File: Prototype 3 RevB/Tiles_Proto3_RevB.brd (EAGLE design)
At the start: 62 parts, among them Q1 DMG3415U-7, U2 MF-DSC-SOT233-MMBT3904, X1 32.768

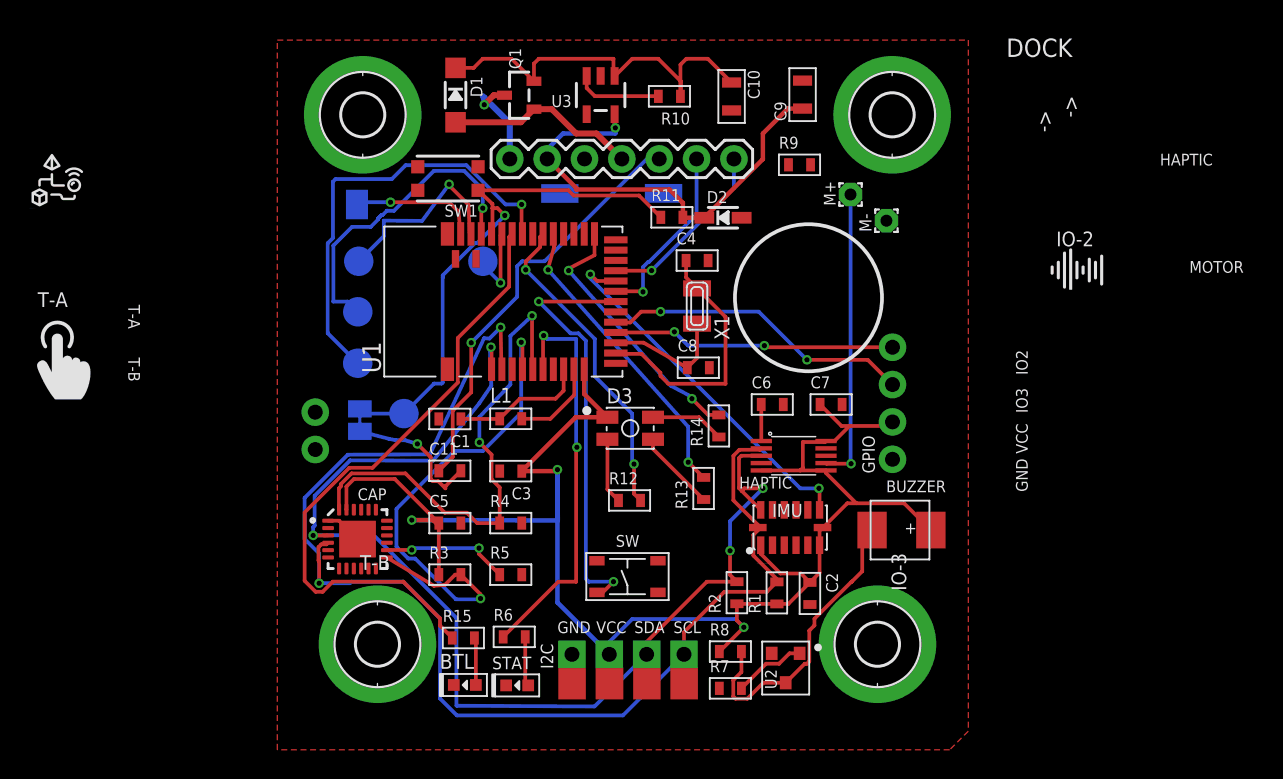
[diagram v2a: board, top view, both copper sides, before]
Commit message: ready for prod
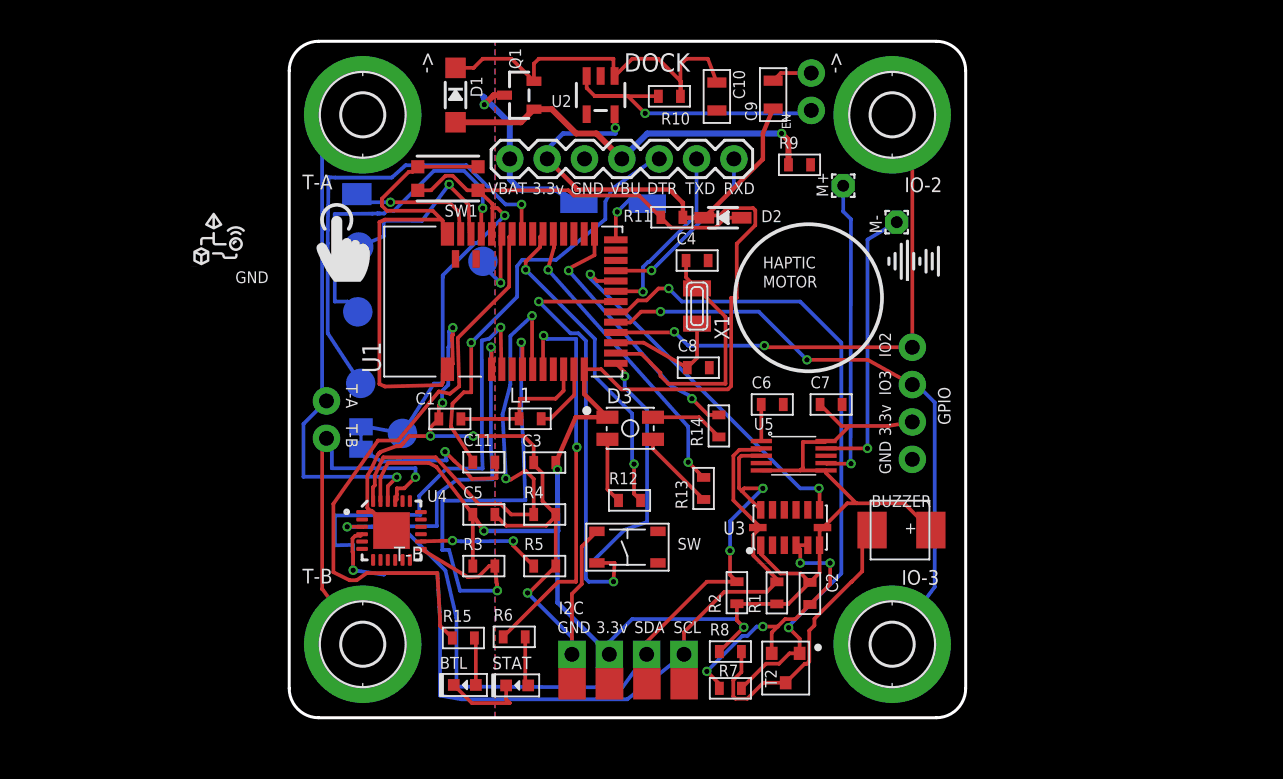
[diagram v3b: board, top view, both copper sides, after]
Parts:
- removed CAP: (no value), cap1188-microbuilder:QFN24_4MM_SMSC
- removed IMU: ADXL345BCCZ-RL, Seeed-OPL-sensor:LGA14-0.8-5.0X3.0MM
- added EN: (no value), SparkFun-Connectors:1X02_NO_SILK
- added T2: MF-DSC-SOT233-MMBT3904, MF_Discrete_Semiconductor:SOT-23-3
- added U4: CAP1188, cap1188-microbuilder:QFN24_4MM_SMSC
- U1: value (none) -> MDBT42Q
- U2: value MF-DSC-SOT233-MMBT3904 -> AP2112; device MF_Discrete_Semiconductor:SOT-23-3 -> microbuilder2:SOT23-5
- U3: value (none) -> ADXL345; device microbuilder2:SOT23-5 -> Seeed-OPL-sensor:LGA14-0.8-5.0X3.0MM
- moved U2 40.9 mm to (18.2, 1.34), turned to 180 degrees
- moved U3 32.1 mm to (31.1, -28.1), turned to 90 degrees
- moved C11 2.38 mm to (10.2, -23.6)
- moved C3 2.38 mm to (14.4, -23.6)
- moved C5 2.38 mm to (10.2, -27.2)
- moved R3 2.38 mm to (10.2, -30.7)
- moved R4 2.38 mm to (14.4, -27.2)
- moved R5 2.38 mm to (14.4, -30.7)
- moved C9 2.00 mm to (29.9, 1.37)
- moved SW 2.00 mm to (20.0, -29.4)
- moved B+ 1.47 mm to (16.7, -6.04)
- moved SWO 1.39 mm to (1.86, -18.3)
- moved RST 1.35 mm to (4.70, -21.7)
- moved GPIO 1.35 mm to (39.4, -15.8)
- moved L1 1.32 mm to (13.4, -20.7)
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- renumbered HAPTIC to U5
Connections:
- removed net N$10: R10.P$2, U3.3
- new net EN: EN.1, R10.P$2, U2.3
- net 3.3V: now also U2.5, U3.1, U3.6, U3.7, U4.23; no longer CAP.23, IMU.1, IMU.6, IMU.7, U3.5
- net BUZZER: now also T2.P$1; no longer U2.P$1
- net CAP-A: now also U4.22; no longer CAP.22
- net CAP-B: now also U4.21; no longer CAP.21
- net CAP-INT: now also U4.13; no longer CAP.13
- net CAP-RES: now also U4.24; no longer CAP.24
- net GND: now also EN.2, T2.P$2, U2.2, U3.4, U3.5, U4.1, U4.THERM; no longer CAP.1, CAP.THERM, IMU.2, IMU.4, IMU.5, U2.P$2
- net IMU-INT: now also U3.8; no longer IMU.8
- net N$13: now also U2.1; no longer U3.1
- net N$3: now also U4.14; no longer CAP.14
- net N$4: now also T2.P$3; no longer U2.P$3
- net SCL: now also U3.14, U4.4; no longer CAP.4, IMU.14
- net SDA: now also U3.13, U4.3; no longer CAP.3, IMU.13
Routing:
- net GND: track 2.52 -> 145.2 mm, vias 0 -> 11
- net BUZZER: track 4.95 -> 45.4 mm, vias 0 -> 2
- net CAP-A: track 0.00 -> 34.8 mm, vias 0 -> 1
- net CAP-B: track 0.00 -> 26.2 mm, vias 0 -> 1
- net EN: track 0.00 -> 21.2 mm, vias 0 -> 1
- net IO-3: track 21.2 -> 41.7 mm
- net N$7: track 0.00 -> 19.3 mm, vias 0 -> 1
- net 3.3V: track 143.8 -> 163.0 mm
- net IO-2: track 19.3 -> 37.0 mm
- net VBUS: track 13.1 -> 27.0 mm, vias 0 -> 1
- net RESET: track 37.5 -> 49.5 mm
- net VBAT: track 7.16 -> 13.8 mm
- net N$10: track 5.93 -> 0.00 mm
- net N$20: track 9.68 -> 12.2 mm
- net BT_LED: track 42.9 -> 41.2 mm
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- added copper zone on layer 16, net GND
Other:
- board outline added: 46 x 46 mm
- board text added: "3.3v"
- board text added: "DTR"
- board text added: "P#3 RevB (2017)"
- board text added: "RXD"
- board text added: "TXD"
- board text added: "VBAT"
- board text added: "VBU"
- board text added: "http://tilestoolkit.io"
- board text added: "simone.mora@ntnu.no"
- board text removed: "Make everyday things interactive http://tilestoolkit.io"
- board text removed: "P#3 RevA (2017)"
- board text removed: "Simone Mora"
- board text removed: "VCC"

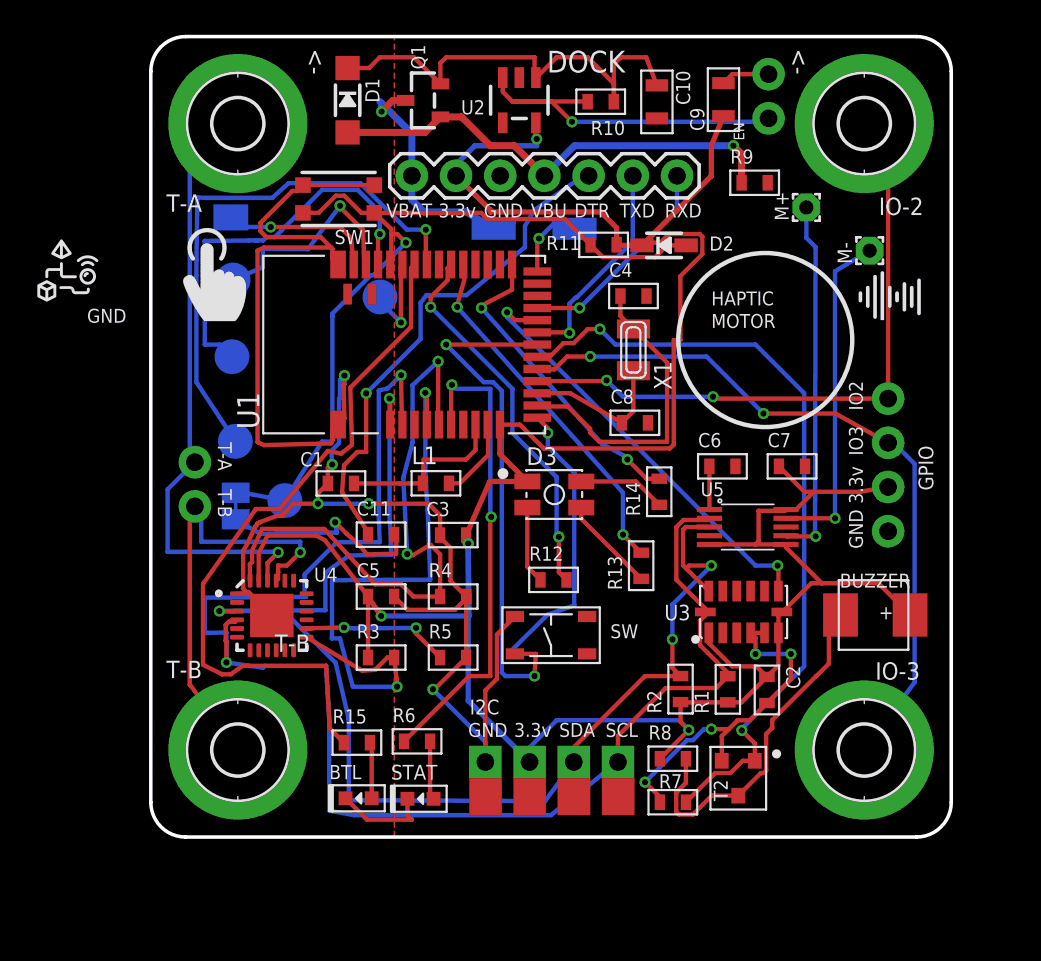
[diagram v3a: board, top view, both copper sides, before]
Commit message: added dock p1rb
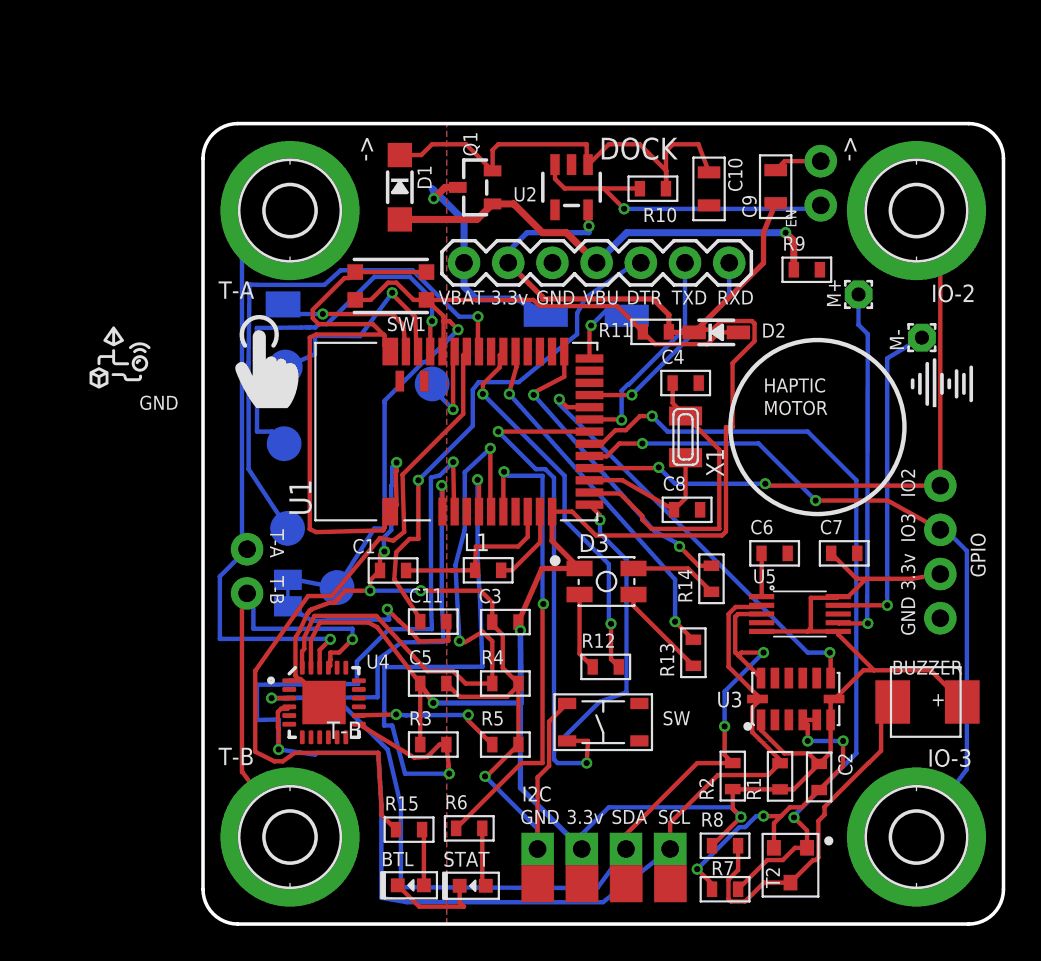
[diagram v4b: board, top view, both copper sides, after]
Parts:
- moved R9 5.83 mm to (34.7, -8.40)
- moved SWCLK 5.83 mm to (4.66, -18.4)
- moved B+ 5.83 mm to (19.7, -11.0)
- moved B- 5.83 mm to (24.4, -11.0)
- moved M- 5.83 mm to (41.3, -12.3)
- moved R11 5.83 mm to (26.0, -12.0)
- moved SW1 5.83 mm to (10.8, -9.33)
- moved BTL 5.83 mm to (11.9, -43.8)
- moved BUZZER 5.83 mm to (41.8, -33.5)
- moved C1 5.83 mm to (10.9, -25.7)
- moved C10 5.83 mm to (29.1, -3.75)
- moved C11 5.83 mm to (13.2, -28.6)
- moved C2 5.83 mm to (35.4, -37.5)
- moved C3 5.83 mm to (17.4, -28.6)
- moved C4 5.83 mm to (27.7, -14.9)
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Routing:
- net EN: track 21.2 -> 19.0 mm

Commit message: values back in sch
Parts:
- C1, C6, C7: value (none) -> 1uF
- C10, C5, C9: value (none) -> 10uF
- C11: value (none) -> 0.1uF
- C2: value (none) -> 100nF
- C4, C8: value (none) -> 22pF
- L1: value (none) -> 10uH
- R1, R11, R2, R3, R4, R7: value (none) -> 10K
- R10, R5, R9: value (none) -> 100K
- R12: value (none) -> 27
- R13, R14: value (none) -> 22
- R15, R6: value (none) -> 330
- R8: value (none) -> 1K

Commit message: re-added part values
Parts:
- C3: value (none) -> 10uF
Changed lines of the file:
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@@
 <attribute name="VOLTAGE" value="" x="10.923" y="-25.6815" size="1.778" layer="27" rot="R180" display="off"/>
 </element>
-<element name="C3" library="MF_Passives" package="C0603" value="" x="17.3749" y="-28.6458" smashed="yes" rot="R180">
+<element name="C3" library="MF_Passives" package="C0603" value="10uF" x="17.3749" y="-28.6458" smashed="yes" rot="R180">
 <attribute name="DIELECTRIC" value="" x="17.3749" y="-28.6458" size="1.778" layer="27" rot="R180" display="off"/>
 <attribute name="HOUSEPART" value="" x="17.3749" y="-28.6458" size="1.778" layer="27" rot="R180" display="off"/>
